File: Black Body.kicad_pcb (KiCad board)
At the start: 2 copper layers, 55.5 x 53.8 mm, 38 parts, among them IC2 MCP96L00T-E_MX, J1 53307-2471, J2 Conn_01x02, J3 Conn_01x04, J5 Conn_02x04_Top_Bottom, J7 Conn_02x03_Top_Bottom

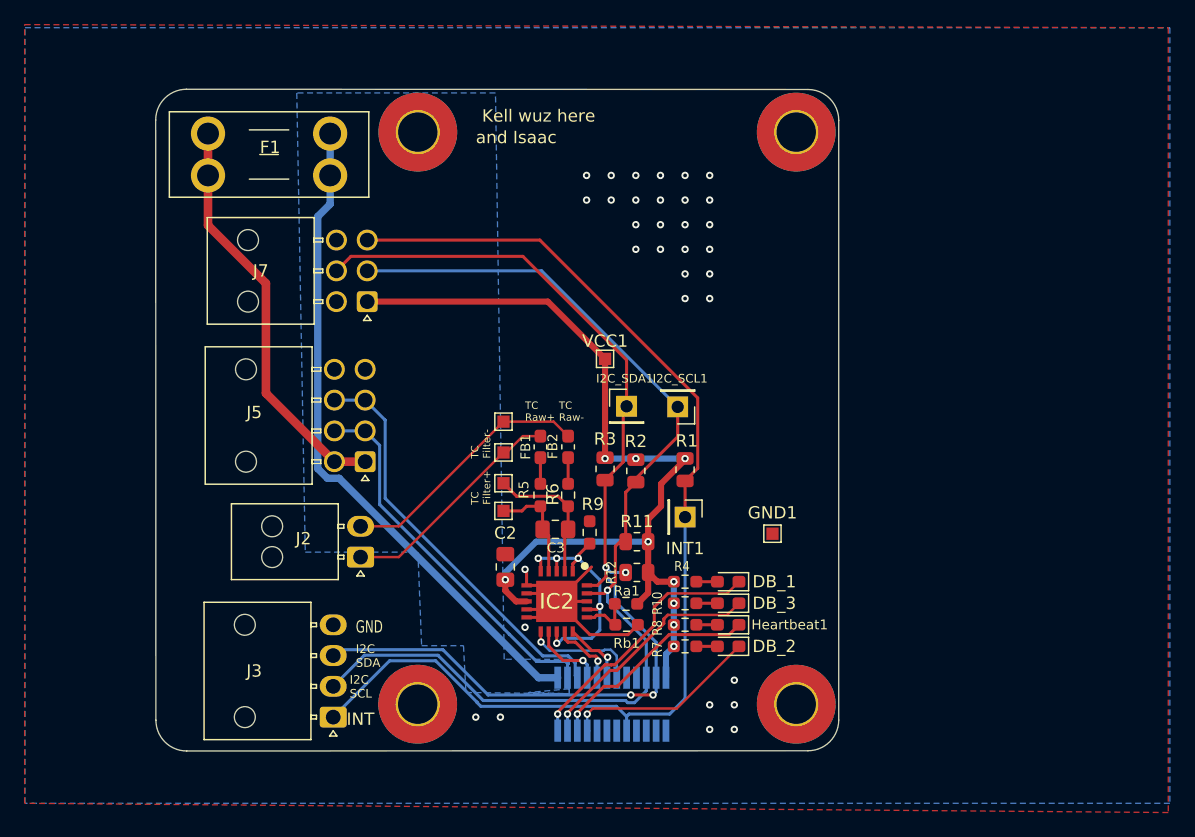
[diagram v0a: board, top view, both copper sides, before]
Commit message: Updated KiCad Sharepoint
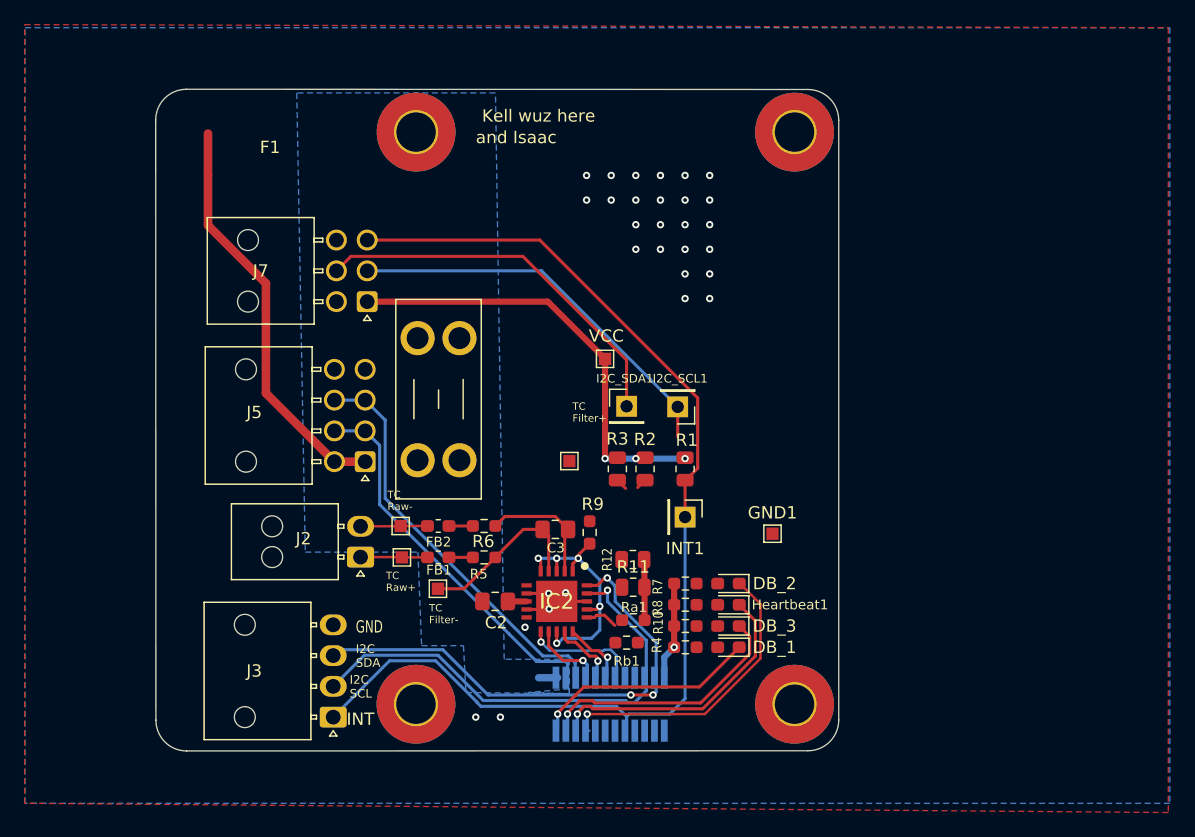
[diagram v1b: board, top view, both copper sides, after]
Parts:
- moved F2 31.5 mm to (95.3, 97.1), turned to 90 degrees
- moved FB2 12.4 mm to (97.0, 102.5), turned to 0 degrees
- moved FB1 12.2 mm to (97.0, 105.0), turned to 0 degrees
- moved TP_TC_2 11.9 mm to (93.9, 102.5)
- moved TP_TC_1 11.9 mm to (94.0, 105.0)
- moved TP_TC_F_1 8.27 mm to (96.9, 107.6)
- moved R6 7.27 mm to (100.7, 102.5), turned to 180 degrees
- moved R5 6.82 mm to (100.7, 105.0), turned to 180 degrees
- moved TP_TC_F_2 5.64 mm to (107.6, 97.2)
- moved DB_1 5.33 mm to (120.5, 112.3)
- moved R4 5.33 mm to (117.0, 112.3)
- moved DB_2 5.10 mm to (120.5, 107.2)
- moved R7 5.10 mm to (117.0, 107.2)
- moved R11 3.71 mm to (112.8, 107.5)
- moved C2 2.92 mm to (101.6, 108.6), turned to 0 degrees
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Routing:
- net +24V: track 54.1 -> 1.55 mm
- net +3V3: track 76.2 -> 50.2 mm, vias 9 -> 4
- net /I2C1_SDA: track 89.6 -> 73.6 mm, vias 4 -> 3
- net /Temp-: track 20.9 -> 5.28 mm
- net /I2C1_SCL: track 88.0 -> 73.5 mm
- net GND: track 20.9 -> 7.12 mm, vias 33 -> 30
- net /Temp+: track 18.7 -> 5.19 mm
- net /DB_Conn_2: track 16.1 -> 24.3 mm
- net Net-(IC2-VIN-): track 8.82 -> 14.2 mm
- net /Heartbeat: track 17.5 -> 22.7 mm
- net /DB_Conn_1: track 21.5 -> 18.5 mm
- net Net-(DB_3-A): track 1.96 -> 0.00 mm
- net Net-(IC2-ADDR): track 4.50 -> 2.68 mm
- net /DB_Conn_3: track 19.3 -> 21.0 mm
- net Net-(DB_2-A): track 1.71 -> 0.00 mm
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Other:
- board text added: "VCC"
